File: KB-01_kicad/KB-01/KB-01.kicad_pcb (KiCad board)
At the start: 6 copper layers, 138 parts, among them IC1 MAX17048G+T10, J1 Conn_01x22_MountingPin, J11 Conn_02x07_Odd_Even, J12 Conn_01x01_Socket, J13 Conn_01x22_MountingPin, J14 Micro_SD_Card_Det, J2 Conn_01x03, J3 USB_C_Receptacle_USB2.0_14P, J4 Conn_01x02_MountingPin, J5 Conn_01x01_Socket, J6 Conn_Coaxial, J8 Bus_M.2_Socket_M, J9 AudioJack3_SwitchTR, Q1 MMBT3904, Q2 2N7002, SW1 Right angle Tact button, SW2 Power button, SW3 RotaryEncoder_Switch_MP, SW4 SW_Push, SW5 SW_Push, U1 BQ25895, U10 AP3441SHE-7B, U11 BMP581, U12 BMI270, U13 SHT40, U14 LIS2MDL, U18 RT9742GGJ5 / NCP380HSN10AAT1G, U2 TS3USB30ERSWR, U3 TLV70430DBVR, U4 TPS61022, U5 TLV773_SOT353, U6 TESEO-LIV4F, U9 ASEK-32.768KHZ-L-R-T

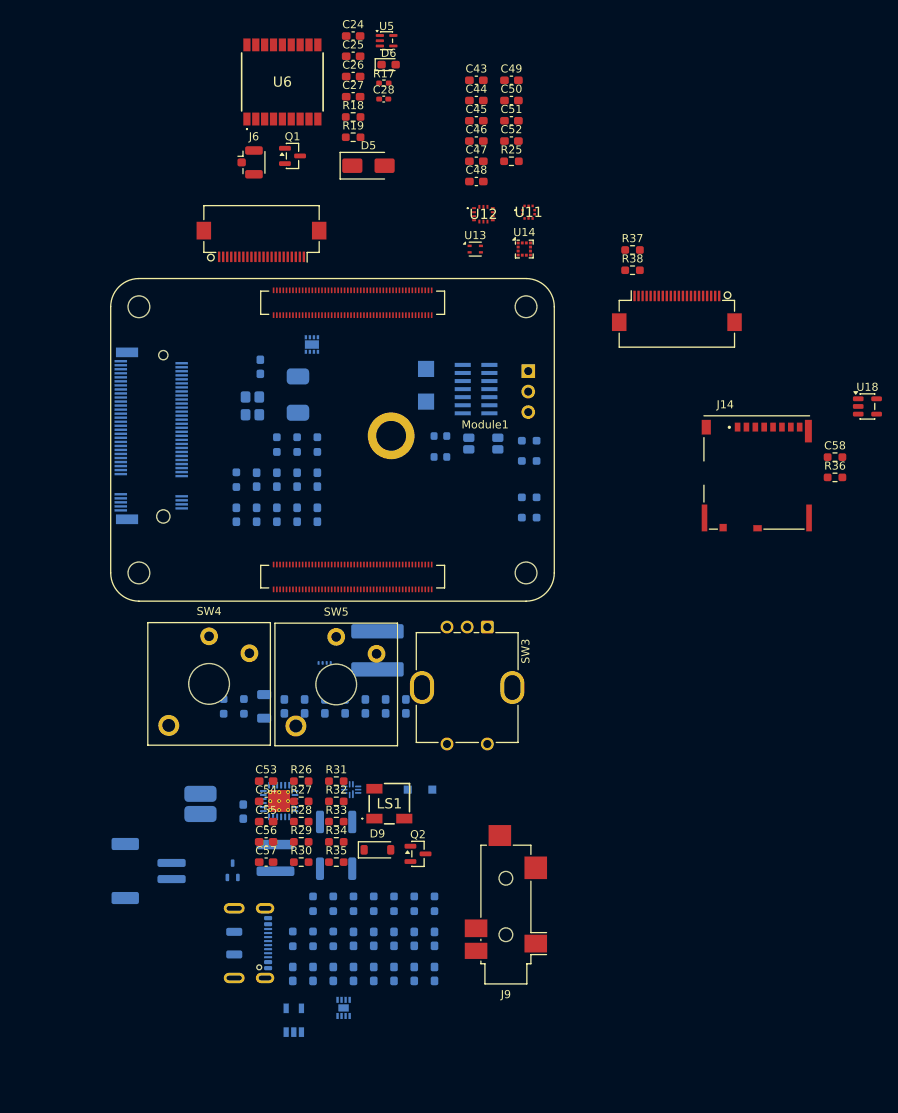
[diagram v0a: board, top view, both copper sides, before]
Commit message: all
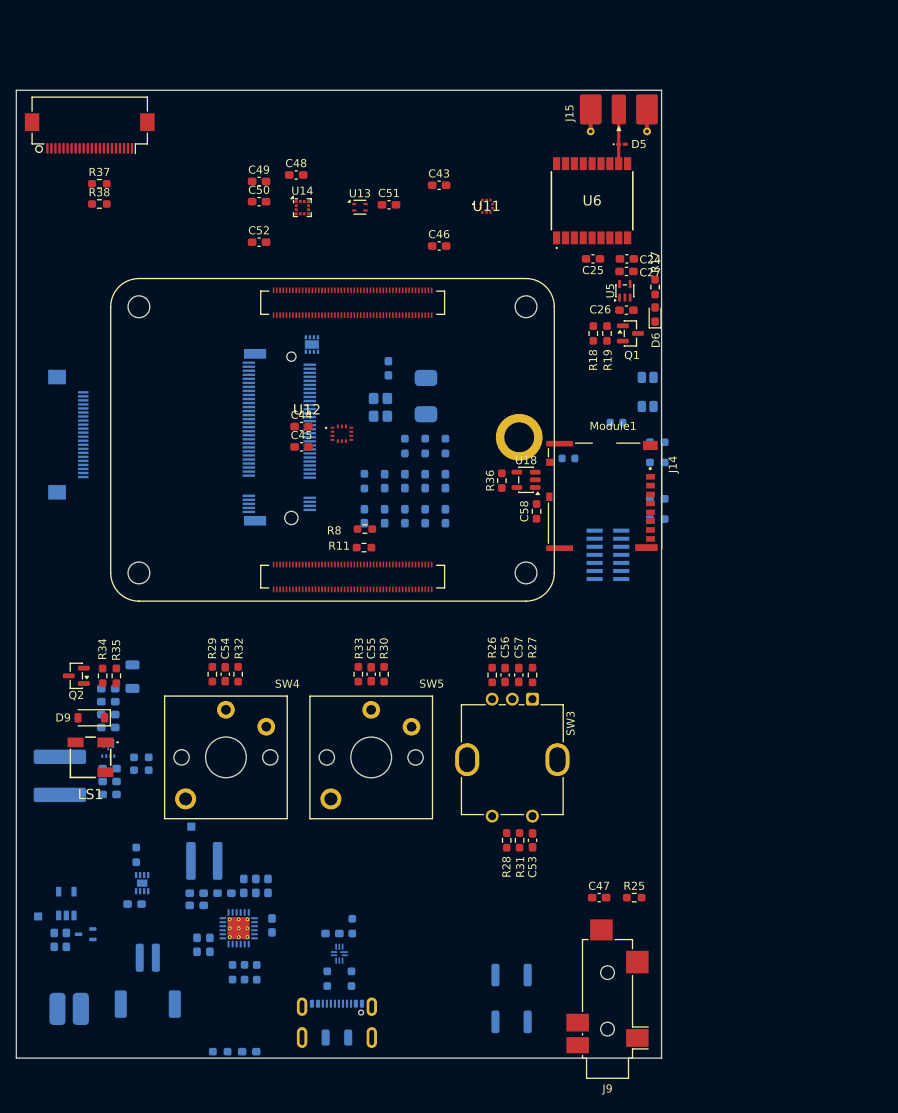
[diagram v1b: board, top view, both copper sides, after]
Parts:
- removed C28: 56pF 50V, Capacitor_SMD:C_0402_1005Metric_Pad0.74x0.62mm_HandSolder
- removed J2: Conn_01x03, Connector_PinHeader_2.54mm:PinHeader_1x03_P2.54mm_Vertical
- removed J6: Conn_Coaxial, Connector_Coaxial:U.FL_Hirose_U.FL-R-SMT-1_Vertical
- removed TP1, TP2: TestPoint, TestPoint:TestPoint_Pad_2.0x2.0mm
- added J15: Conn_Coaxial, Connector_Coaxial:SMA_Molex_73251-2120_EdgeMount_Horizontal, F.Cu at (138.3, 38.8)
- D5: footprint Diode_SMD:D_SMA -> Diode_SMD:D_0201_0603Metric_Pad0.64x0.40mm_HandSolder
- J1: moved to B.Cu
- R11, R8: moved to F.Cu
- R17: footprint Resistor_SMD:R_0402_1005Metric_Pad0.72x0.64mm_HandSolder -> Resistor_SMD:R_0603_1608Metric_Pad0.98x0.95mm_HandSolder
- SW4, SW5: footprint PCM_Switch_Keyboard_Kailh:SW_Kailh_Choc_V2 -> PCM_Switch_Keyboard_Kailh:SW_Kailh_Choc_V1V2_1.00u
- moved C47 92.6 mm to (135.9, 136.8)
- moved R25 92.6 mm to (140.2, 136.8)
- moved J13 76.1 mm to (72.7, 42.0), turned to 180 degrees
- moved R37 66.6 mm to (73.9, 48.3)
- moved R38 66.6 mm to (73.9, 50.8)
- moved TP4 48.4 mm to (66.3, 139.1), turned to 0 degrees
- moved Q2 47.8 mm to (71.0, 109.3), turned to 180 degrees
- moved Q1 47.3 mm to (139.7, 66.8)
- moved R8 47.3 mm to (106.8, 91.1), turned to 180 degrees
- moved C44 45.9 mm to (99.0, 78.4)
- moved C45 45.9 mm to (99.0, 80.9)
- moved D6 45.3 mm to (142.8, 64.5), turned to 90 degrees
- moved C26 44.6 mm to (139.2, 64.0)
- moved R11 44.2 mm to (106.7, 93.4), turned to 180 degrees
- moved C24 43.8 mm to (139.3, 57.6)
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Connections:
- U6 pad 11: Net-(U6-RF_IN) -> Net-(D5-A1)
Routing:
- net Net-(D5-A1): track 0.00 -> 6.75 mm
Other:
- board outline added: 80 x 120 mm
